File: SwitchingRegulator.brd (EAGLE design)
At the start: 84.6 x 78.7 mm, 30 parts, among them J1 APP_2POS_CONFIG5V_HORIZ, J2 APP_2POS_CONFIG5V_HORIZ, J3 APP_2POS_CONFIG5V_HORIZ, Q2 Q_CSD18532KCSPCB, Q3 Q_CSD18532KCSPCB, U1 OKI-78SR-5/1.5-W36HC

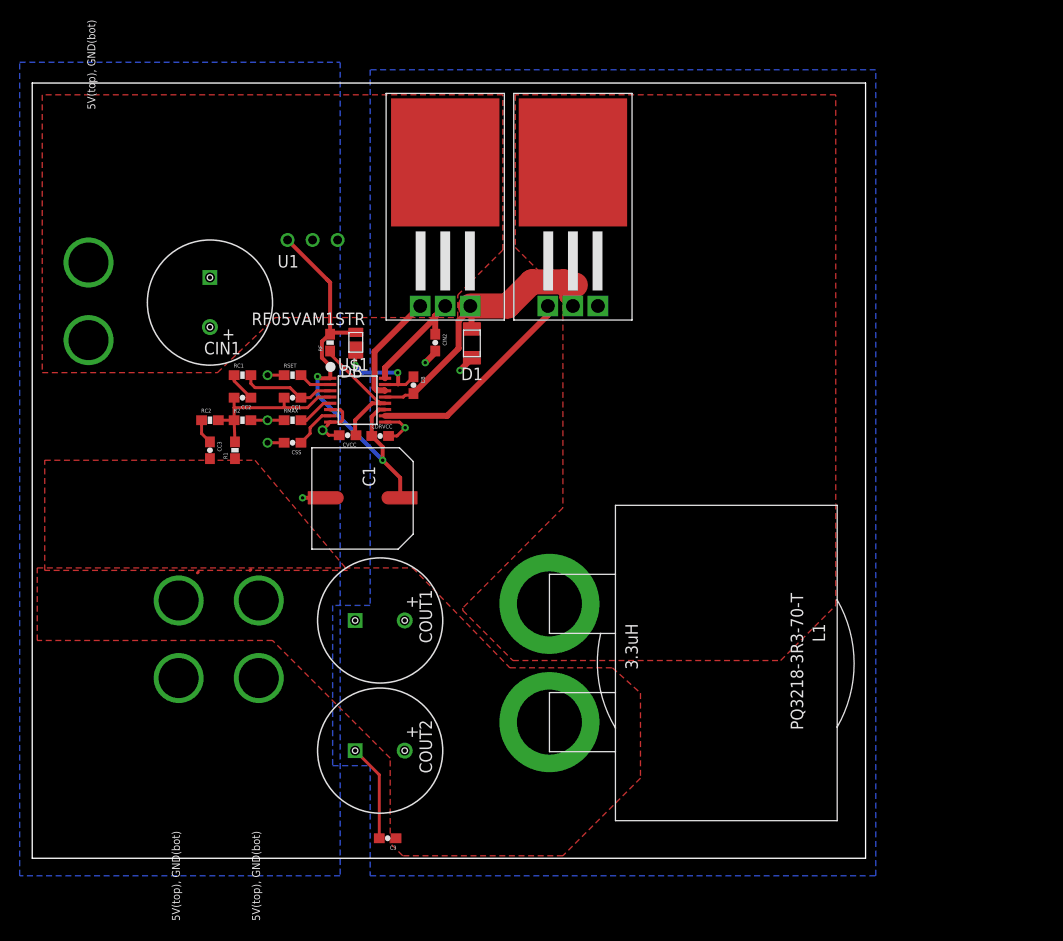
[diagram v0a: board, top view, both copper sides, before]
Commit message: New layout, do power power path
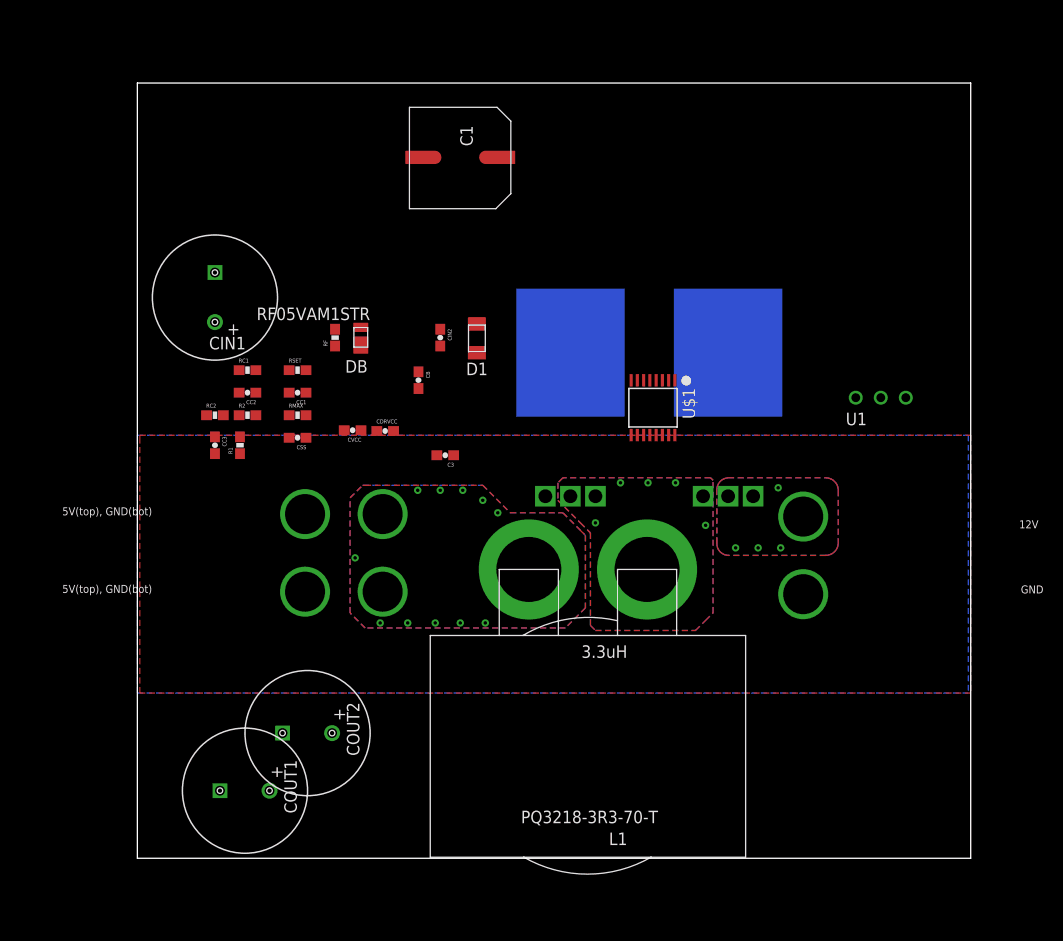
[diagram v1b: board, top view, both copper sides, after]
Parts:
- removed J3: APP_2POS_CONFIG5V_HORIZ, MRDT-Connectors:APP45_5V_HORIZ_CONFIG
- added J4: APP_2POS_CONFIG12V_HORIZ, MRDT-Connectors:APP45_12V_HORIZ_CONFIG
- moved U1 59.8 mm to (78.2, 46.7)
- moved J1 49.2 mm to (-10.9, 31.0), turned to 0 degrees
- moved C3 39.3 mm to (31.5, 40.9)
- moved J2 38.2 mm to (-10.9, 23.1), turned to 0 degrees
- moved C1 35.9 mm to (33.0, 71.1)
- moved Q2 34.6 mm to (60.2, 51.3), flipped to the bottom
- moved U$1 30.0 mm to (52.6, 45.7), turned to 180 degrees
- moved COUT1 22.1 mm to (11.2, 6.86)
- moved Q3 19.3 mm to (44.2, 51.3), flipped to the bottom
- moved L1 18.7 mm to (62.0, 22.6), turned to 180 degrees
- moved COUT2 7.58 mm to (17.5, 12.7)
- moved CC1 0.72 mm to (16.5, 47.2)
- moved RSET 0.72 mm to (16.5, 49.5)
- moved CIN1 0.72 mm to (8.13, 56.9)
- moved CB 0.72 mm to (28.8, 48.5)
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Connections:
- net GND: now also J4.GND; no longer J3.GND
- net VBATT: now also J4.12V; no longer J3.5V
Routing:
- net N$15: track 43.6 -> 0.00 mm, vias 2 -> 0
- net GND: track 33.1 -> 0.00 mm, vias 8 -> 0
- net N$17: track 30.4 -> 0.00 mm
- net N$16: track 21.7 -> 0.00 mm
- net N$11: track 17.3 -> 0.00 mm
- net N$13: track 12.8 -> 0.00 mm
- net VBATT: track 11.7 -> 0.00 mm
- net N$2: track 11.4 -> 0.00 mm
- net N$1: track 10.1 -> 0.00 mm, vias 2 -> 0
- net N$7: track 9.79 -> 0.00 mm
- net N$6: track 4.46 -> 0.00 mm
- net N$4: track 3.69 -> 0.00 mm
- net N$3: track 3.64 -> 0.00 mm
- net N$9: track 2.99 -> 0.00 mm
- net N$10: track 2.55 -> 0.00 mm
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- added copper zone on layer 1, net GND
- added copper zone on layer 16, net N$17
- added copper zone on layer 16, net VBATT1
- added copper zone on layer 16, net VOUT12+
